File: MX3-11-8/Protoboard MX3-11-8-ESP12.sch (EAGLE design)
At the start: 638 parts, among them J1 DCJ0202, X3 RJ45

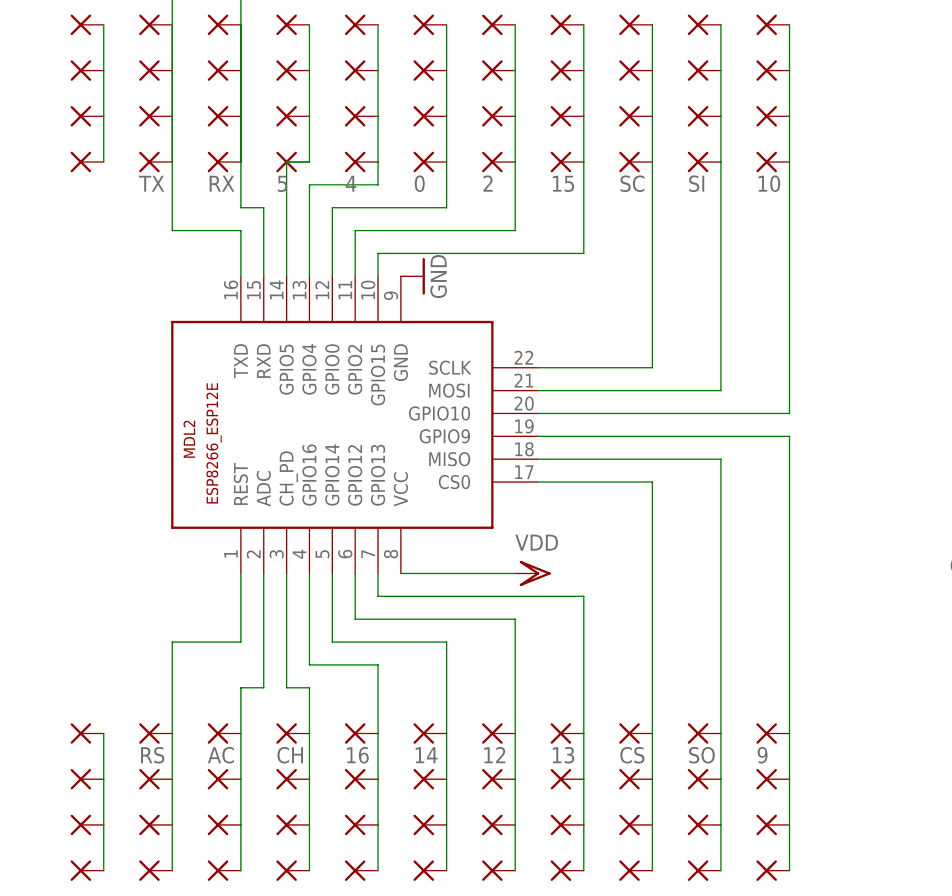
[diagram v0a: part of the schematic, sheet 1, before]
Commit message: Update esp component and usb
test
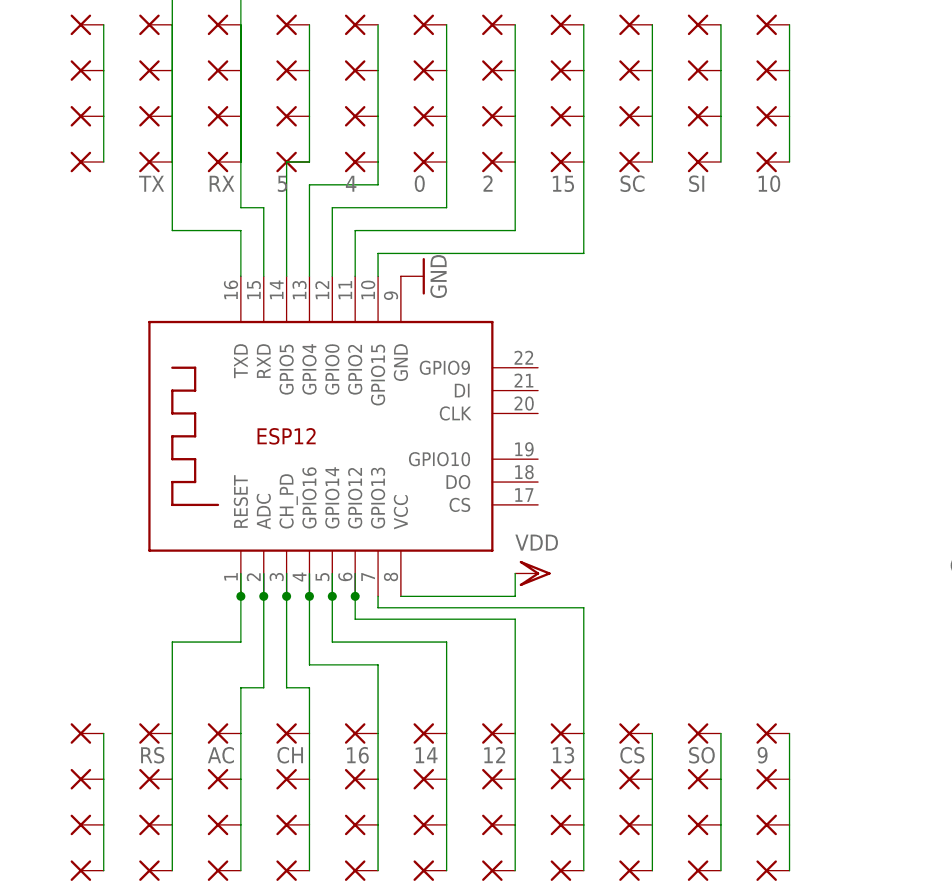
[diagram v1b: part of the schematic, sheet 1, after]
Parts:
- removed MDL2: (no value), ESP8266-ESP12E:ESP8266-12EESP8266-ESP12E
- added X1: ESP-12E, microbuilder:ESP-12E
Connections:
- removed net N$58: MDL2.MOSI, PAD762.P, PAD763.P, PAD764.P, PAD765.P
- removed net N$85: MDL2.GPIO10, PAD766.P, PAD767.P, PAD768.P, PAD769.P
- new net N$29: PAD762.P, PAD763.P, PAD764.P, PAD765.P
- new net N$30: PAD766.P, PAD767.P, PAD768.P, PAD769.P
- net GND: now also X1.GND; no longer MDL2.GND
- net N$113: now also X1.CH_PD; no longer MDL2.CH_PD
- net N$121: now also X1.GPIO13; no longer MDL2.GPIO13
- net N$122: no longer MDL2.MISO
- net N$47: now also X1.GPIO5; no longer MDL2.GPIO5
- net N$48: now also X1.GPIO4; no longer MDL2.GPIO4
- net N$52: now also X1.GPIO0; no longer MDL2.GPIO0
- net N$53: now also X1.GPIO2; no longer MDL2.GPIO2
- net N$54: now also X1.GPIO15; no longer MDL2.GPIO15
- net N$55: no longer MDL2.SCLK
- net N$56: now also X1.GPIO14; no longer MDL2.GPIO14
- net N$57: no longer MDL2.CS0
- net N$86: no longer MDL2.GPIO9
- net N$87: now also X1.RESET; no longer MDL2.REST
- net N$88: now also X1.ADC; no longer MDL2.ADC
- net N$90: now also X1.GPIO16; no longer MDL2.GPIO16
- net N$91: now also X1.GPIO12; no longer MDL2.GPIO12
- net RX: now also X1.RXD; no longer MDL2.RXD
- net TX: now also X1.TXD; no longer MDL2.TXD
- net VDD: now also X1.VCC; no longer MDL2.VCC
